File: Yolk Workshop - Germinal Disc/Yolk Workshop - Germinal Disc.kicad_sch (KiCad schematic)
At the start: 5 parts

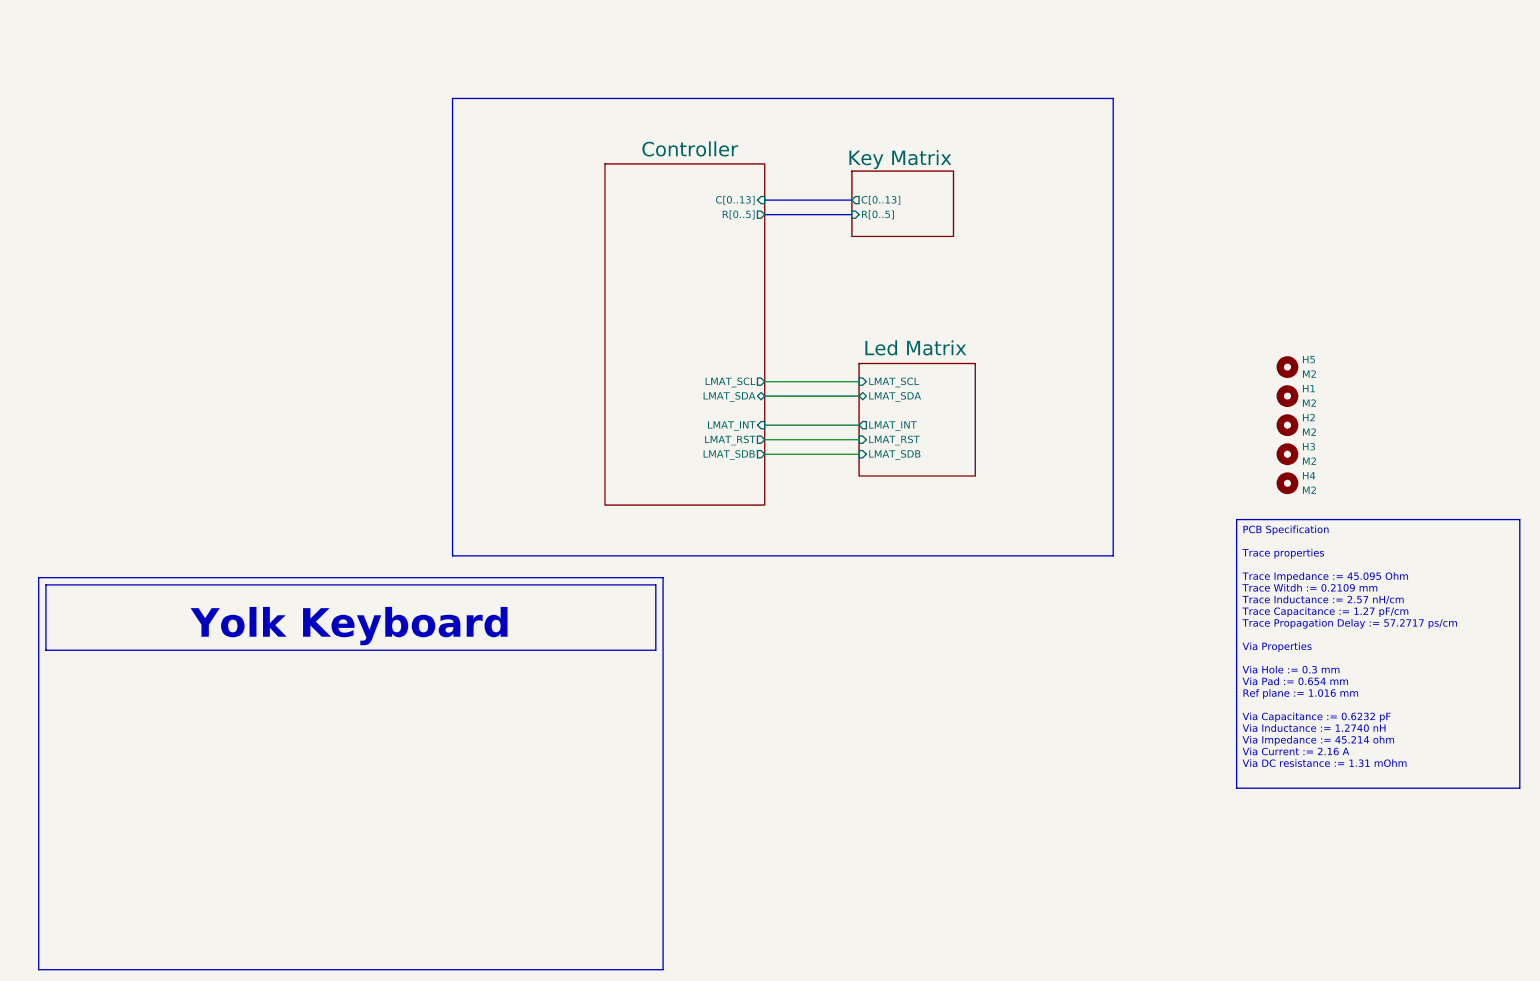
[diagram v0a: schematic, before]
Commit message: updates to HIP and Controller design
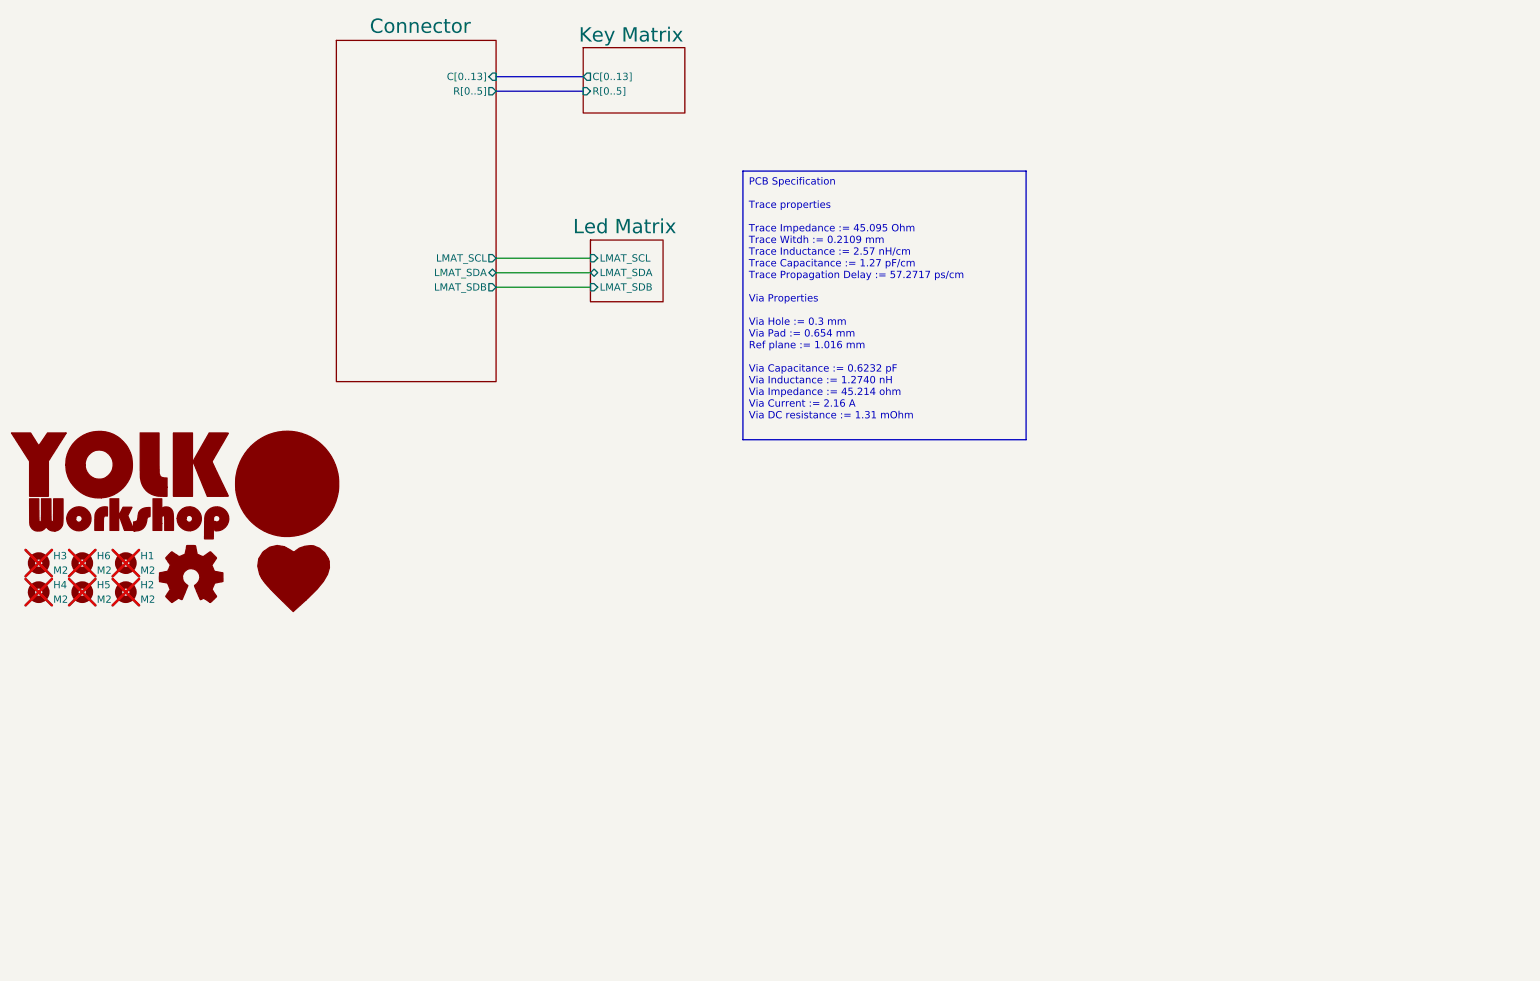
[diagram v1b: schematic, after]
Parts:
- added H6: M2, MountingHole:MountingHole_2.2mm_M2, symbol Mechanical:MountingHole
- H1, H2, H3, H4, H5: now not fitted
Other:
- sheet Controller renamed Connector
- sheet Connector ports: added none; removed LMAT_INT, LMAT_RST
- sheet Led Matrix ports: added none; removed LMAT_INT, LMAT_RST
